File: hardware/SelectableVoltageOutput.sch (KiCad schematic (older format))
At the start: 8 parts, among them J1601 Power_select, Q1601 ZXTN25050DFHTA, Q1602 ZXTN25050DFHTA

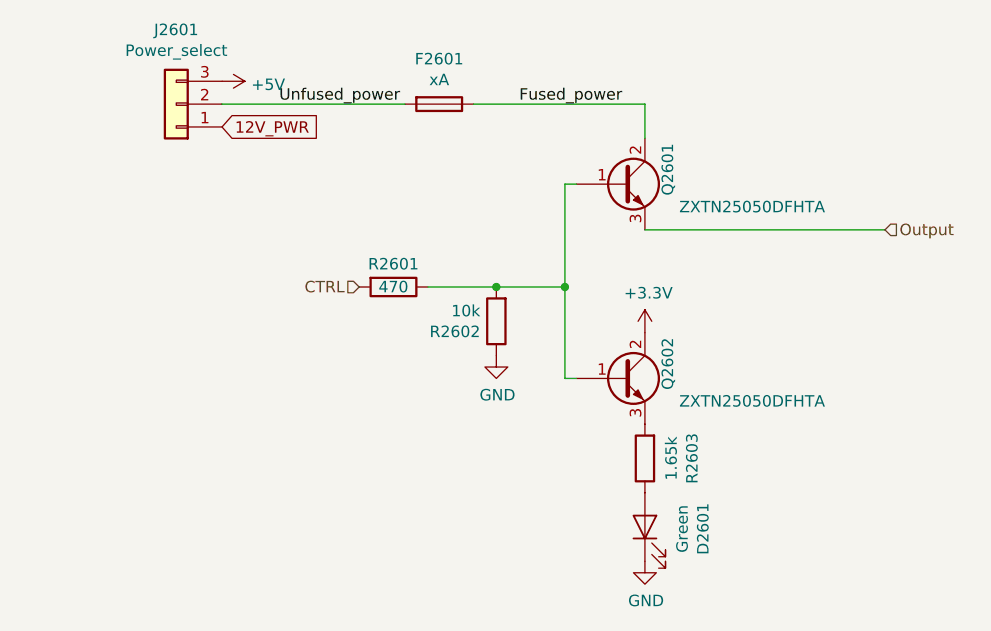
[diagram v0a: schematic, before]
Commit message: Outputs now uses MOSFETs
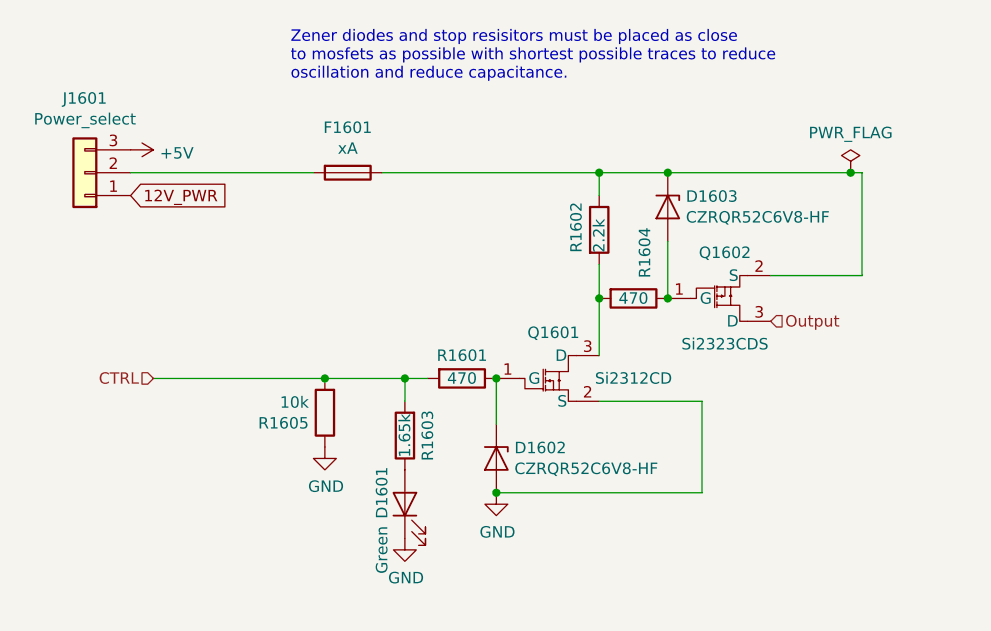
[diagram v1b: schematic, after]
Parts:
- removed Q1601, Q1602: ZXTN25050DFHTA, Package_TO_SOT_SMD:SOT-23, symbol Device:Q_NPN_BCE
- added D1602, D1603: CZRQR52C6V8-HF, Diode_SMD:D_0402_1005Metric, symbol Device:D_Zener
- added Q1601: Si2312CD, Package_TO_SOT_SMD:SOT-23, symbol PerMalmberg:Si2312CD
- added Q1602: Si2323CDS, Package_TO_SOT_SMD:SOT-23, symbol PerMalmberg:Si2323CDS
- added R1604: 470, Resistor_SMD:R_0805_2012Metric, symbol Device:R
- added R1605: 10k, Resistor_SMD:R_0805_2012Metric, symbol Device:R
- R1602: value 10k -> 2.2k; footprint Resistor_SMD:R_0805_2012Metric -> (none)
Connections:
- net CTRL: now also R1603.2, R1605.2
- net GND: now also D1602.2 (A), Q1601.2 (S), R1605.1; no longer R1602.1
- net Output: now also Q1602.3 (D)
- net at R1601.1: now also D1602.1 (K), Q1601.1 (G); no longer R1602.2
- net Fused_power: no longer names the net of F1601.1
- net Fused_power: now also R1602.1, D1603.1 (K), Q1602.2 (S)
- net Unfused_power: no longer names the net of F1601.2, J1601.2 (Pin_2)
- new net: Q1601.3 (D), R1602.2, R1604.2
- new net: D1603.2 (A), Q1602.1 (G), R1604.1
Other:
- note added: "Zener diodes and stop resisitors must be placed as close\nto mosfets as possible with shortest possible traces to reduce\noscillation and reduce capacitance."
- moved on the sheet: D1601, F1601, J1601, R1603

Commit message: Preparing to replicate layout for outputs.
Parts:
- F1601: footprint Fuse:Fuseholder_TR5_Littlefuse_No560_No460 -> Fuse:Fuseholder_TR5_Littelfuse_No560_No460
- R1602: footprint (none) -> Resistor_SMD:R_0805_2012Metric
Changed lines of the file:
@@
 F 0 "F1601" V 2153 1800 50  0000 C CNN
 F 1 "xA" V 2244 1800 50  0000 C CNN
-F 2 "Fuse:Fuseholder_TR5_Littlefuse_No560_No460" V 2280 1800 50  0001 C CNN
+F 2 "Fuse:Fuseholder_TR5_Littelfuse_No560_No460" V 2280 1800 50  0001 C CNN
 F 3 "https://www.mouser.se/ProductDetail/Littelfuse/56000001019?qs=sGAEpiMZZMtRmoYvq3OwzKEcK5xXAR8uiSqvDZfRA1w%3d" H 2350 1800 50  0001 C CNN
 	1    2350 1800
@@
 F 0 "R1602" V 3350 1950 50  0000 L CNN
 F 1 "2.2k" V 3450 1950 50  0000 L CNN
-F 2 "" V 3380 2050 50  0001 C CNN
-F 3 "~" H 3450 2050 50  0001 C CNN
+F 2 "Resistor_SMD:R_0805_2012Metric" V 3380 2050 50  0001 C CNN
+F 3 "https://www.mouser.se/ProductDetail/667-ERA-6AED222V" H 3450 2050 50  0001 C CNN
 	1    3450 2050
 	1    0    0    -1
